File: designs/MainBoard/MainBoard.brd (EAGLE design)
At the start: 89 x 37 mm, 6 parts

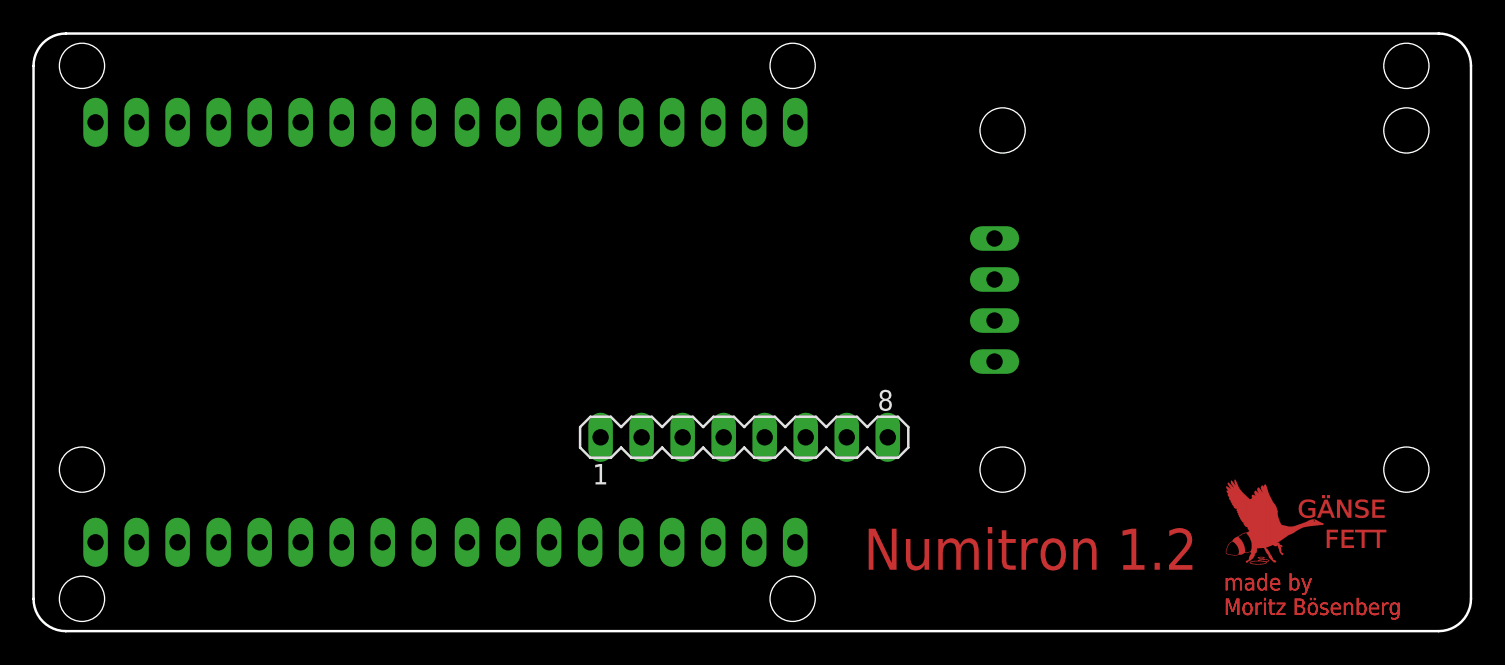
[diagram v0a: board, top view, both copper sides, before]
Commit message: finished mainboard
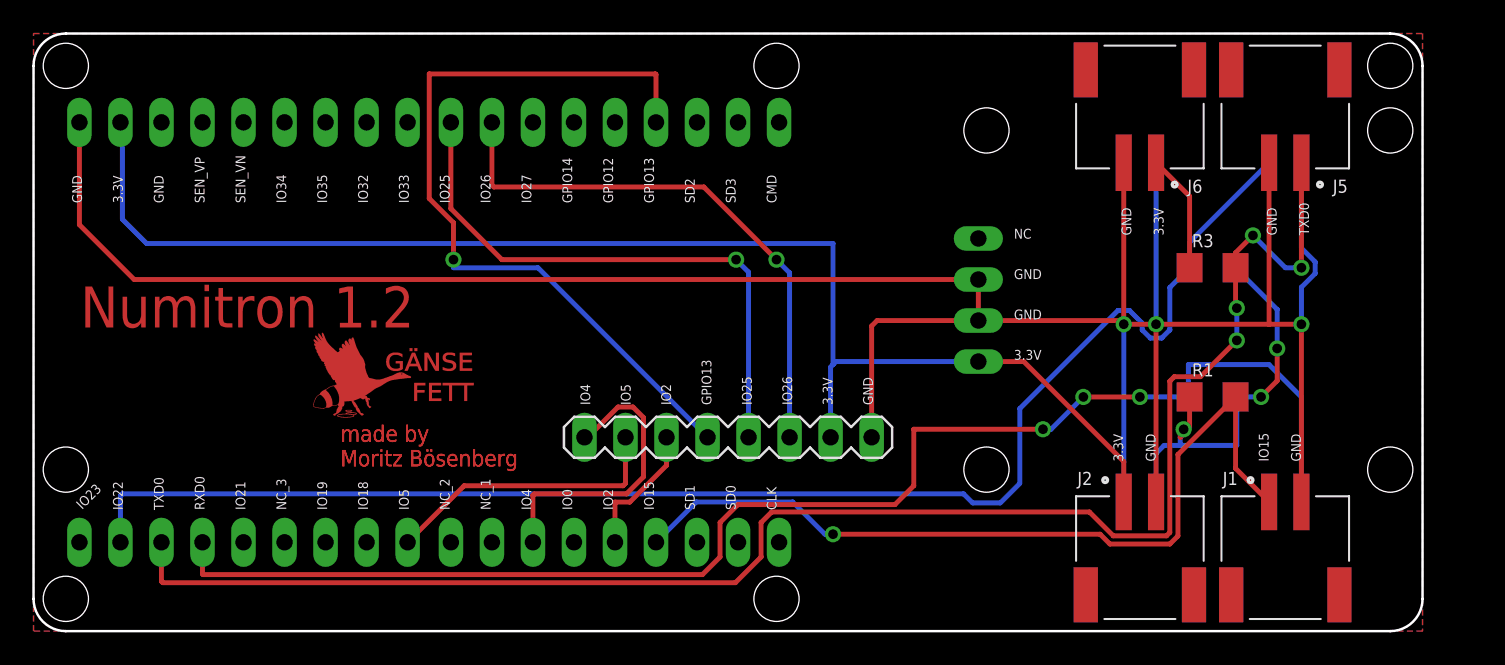
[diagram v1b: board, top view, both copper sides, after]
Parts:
- removed SV1: (no value), con-lstb:MA08-1
- added J1, J2, J3, J4, J5, J6, J7, J8: S2B-PH-SM4, CommonParts:JST_S2B-PH-SM4-TB(LF)(SN)
- added R1, R2, R3, R4: (no value), CommonParts:R1206
- added SV4: (no value), CommonParts:MA08-1
- moved JP1 1.00 mm to (58.5, 20.5)
- moved SV2 1.00 mm to (36.0, 5.50)
- moved SV3 1.00 mm to (13.0, 5.50)
- moved SV5 1.00 mm to (13.0, 31.5)
- moved SV6 1.00 mm to (36.0, 31.5)
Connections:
- net 3.3V: now also J2.1, J4.1, J6.1, J8.1, R1.1, R2.1, R3.1, R4.1, SV4.7; no longer SV1.7
- net GND: now also J1.2, J2.2, J3.2, J4.2, J5.2, J6.2, J7.2, J8.2, SV4.8; no longer SV1.8
- net GPIO13: now also SV4.4; no longer SV1.4
- net IO15: now also J1.1, R1.2
- net IO2: now also SV4.3; no longer SV1.3
- net IO22: now also J7.1, R4.2
- net IO25: now also SV4.5; no longer SV1.5
- net IO26: now also SV4.6; no longer SV1.6
- net IO4: now also SV4.1; no longer SV1.1
- net IO5: now also SV4.2; no longer SV1.2
- net RXD0: now also J3.1, R2.2
- net TXD0: now also J5.1, R3.2
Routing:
- net GND: track 0.00 -> 173.4 mm, vias 0 -> 3
- net 3.3V: track 0.00 -> 119.9 mm, vias 0 -> 3
- net TXD0: track 0.00 -> 100.5 mm, vias 0 -> 4
- net IO22: track 0.00 -> 89.8 mm
- net RXD0: track 0.00 -> 87.3 mm, vias 0 -> 3
- net IO15: track 0.00 -> 52.1 mm, vias 0 -> 1
- net GPIO13: track 0.00 -> 49.7 mm, vias 0 -> 1
- net IO25: track 0.00 -> 35.6 mm, vias 0 -> 1
- net IO26: track 0.00 -> 34.7 mm, vias 0 -> 1
- net IO4: track 0.00 -> 18.6 mm
- net IO5: track 0.00 -> 17.9 mm
- net IO2: track 0.00 -> 8.36 mm
- added copper zone on layer 1, net GND
- added copper zone on layer 16, net GND
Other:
- board size 89 x 37 mm -> 86 x 37 mm
- board text added: "3.3V"
- board text added: "CLK"
- board text added: "CMD"
- board text added: "GND"
- board text added: "GPIO12"
- board text added: "GPIO13"
- board text added: "GPIO14"
- board text added: "IO0"
- board text added: "IO15"
- board text added: "IO18"
- board text added: "IO19"
- board text added: "IO2"
- board text added: "IO21"
- board text added: "IO22"
- board text added: "IO23"
- board text added: "IO25"
- board text added: "IO26"
- board text added: "IO27"
- board text added: "IO32"
- board text added: "IO33"
- board text added: "IO34"
- board text added: "IO35"
- board text added: "IO4"
- board text added: "IO5"
- board text added: "NC"
- board text added: "NC_1"
- board text added: "NC_2"
- board text added: "NC_3"
- board text added: "RXD0"
- board text added: "SD0"
- board text added: "SD1"
- board text added: "SD2"
- board text added: "SD3"
- board text added: "SEN_VN"
- board text added: "SEN_VP"
- board text added: "TXD0"

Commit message: added last design tunes
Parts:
- R1, R2, R3, R4: value (none) -> 10K
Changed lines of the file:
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@@
 <setting verticaltext="up"/>
 </settings>
-<grid distance="0.5" unitdist="mm" unit="mm" style="lines" multiple="1" display="no" altdistance="5" altunitdist="mil" altunit="mil"/>
+<grid distance="0.1" unitdist="mm" unit="mm" style="lines" multiple="1" display="no" altdistance="5" altunitdist="mil" altunit="mil"/>
 <layers>
 <layer number="1" name="Top" color="4" fill="1" visible="yes" active="yes"/>
@@
 </class>
 </classes>
-<designrules name="default *">
+<designrules name="Main_1">
 <description language="de">&lt;b&gt;EAGLE Design Rules&lt;/b&gt;
 &lt;p&gt;
@@
 <param name="mdViaViaSameLayer" value="6mil"/>
 <param name="mnLayersViaInSmd" value="2"/>
-<param name="mdCopperDimension" value="20mil"/>
+<param name="mdCopperDimension" value="10mil"/>
 <param name="mdDrill" value="6mil"/>
 <param name="mdSmdStop" value="0mil"/>
@@
 <attribute name="PACKAGE" value="None" x="68.5" y="29" size="1.778" layer="28" rot="MR180" display="off"/>
 </element>
-<element name="R1" library="CommonParts" package="R1206" package3d_urn="urn:adsk.eagle:package:23540/2" value="" x="73" y="14.5" smashed="yes">
+<element name="R1" library="CommonParts" package="R1206" package3d_urn="urn:adsk.eagle:package:23540/2" value="10K" x="73" y="14.5" smashed="yes">
 <attribute name="NAME" x="71.73" y="15.77" size="0.8128" layer="25"/>
-<attribute name="VALUE" x="71.73" y="11.96" size="1.27" layer="27"/>
+<attribute name="VALUE" x="71.73" y="12.46" size="0.8128" layer="27"/>
 </element>
-<element name="R2" library="CommonParts" package="R1206" package3d_urn="urn:adsk.eagle:package:23540/2" value="" x="73" y="14.5" smashed="yes" rot="MR0">
+<element name="R2" library="CommonParts" package="R1206" package3d_urn="urn:adsk.eagle:package:23540/2" value="10K" x="73" y="14.5" smashed="yes" rot="MR0">
 <attribute name="NAME" x="74.27" y="15.77" size="0.8128" layer="26" rot="MR0"/>
-<attribute name="VALUE" x="74.27" y="11.96" size="1.27" layer="28" rot="MR0"/>
+<attribute name="VALUE" x="74.27" y="12.46" size="0.8128" layer="28" rot="MR0"/>
 </element>
-<element name="R3" library="CommonParts" package="R1206" package3d_urn="urn:adsk.eagle:package:23540/2" value="" x="73" y="22.5" smashed="yes">
+<element name="R3" library="CommonParts" package="R1206" package3d_urn="urn:adsk.eagle:package:23540/2" value="10K" x="73" y="22.5" smashed="yes">
 <attribute name="NAME" x="71.73" y="23.77" size="0.8128" layer="25"/>
-<attribute name="VALUE" x="71.73" y="19.96" size="1.27" layer="27"/>
+<attribute name="VALUE" x="71.73" y="20.46" size="0.8128" layer="27"/>
 </element>
-<element name="R4" library="CommonParts" package="R1206" package3d_urn="urn:adsk.eagle:package:23540/2" value="" x="73" y="22.5" smashed="yes" rot="MR0">
+<element name="R4" library="CommonParts" package="R1206" package3d_urn="urn:adsk.eagle:package:23540/2" value="10K" x="73" y="22.5" smashed="yes" rot="MR0">
 <attribute name="NAME" x="74.27" y="23.77" size="0.8128" layer="26" rot="MR0"/>
-<attribute name="VALUE" x="74.27" y="19.96" size="1.27" layer="28" rot="MR0"/>
+<attribute name="VALUE" x="73.77" y="20.46" size="0.8128" layer="28" rot="MR0"/>
 </element>
 <element name="SV4" library="CommonParts" package="MA08-1" package3d_urn="urn:adsk.eagle:package:8343/1" value="" x="43" y="12" smashed="yes">
